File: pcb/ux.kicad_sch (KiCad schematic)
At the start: 41 parts, among them J5 Conn_01x40, J7 GameBoy_LinkPort, J8 Conn_01x02, SW12 A, SW13 B, SW14 START, SW15 SELECT, SW2 BOOT, SW3 RESET, SW4 UP, SW5 DOWN, SW6 LEFT, SW7 RIGHT, U5 APA2502, U7 ICM-42670-P, U8 TCA9535RTWR

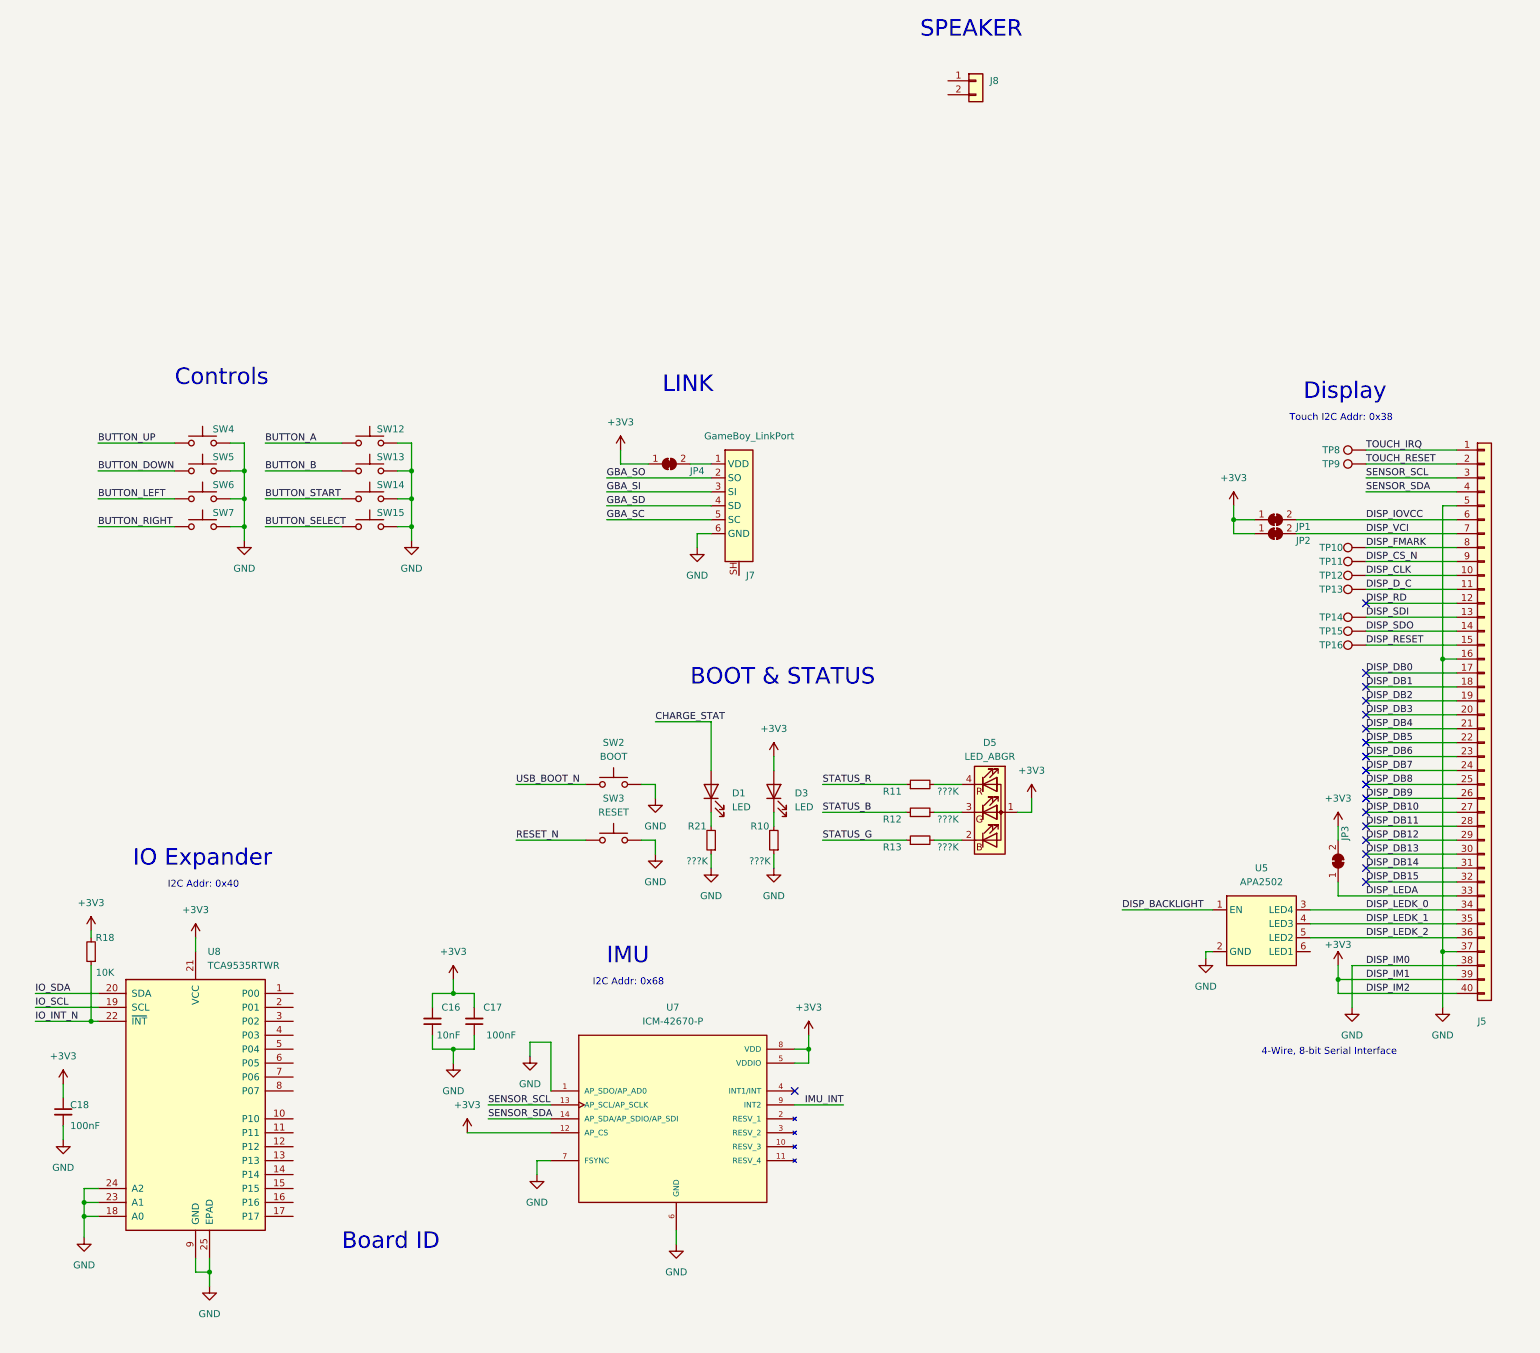
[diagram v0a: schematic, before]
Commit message: pcb: Update schematic to WIP6
Change-Id: I9e9f727ad2774ee986f2f97450dc509901129aec
Reviewed-on: https://pigweed-review.googlesource.com/c/pigweed/kudzu/+/169650
Reviewed-by: Anthony DiGirolamo <tonymd@google.com>
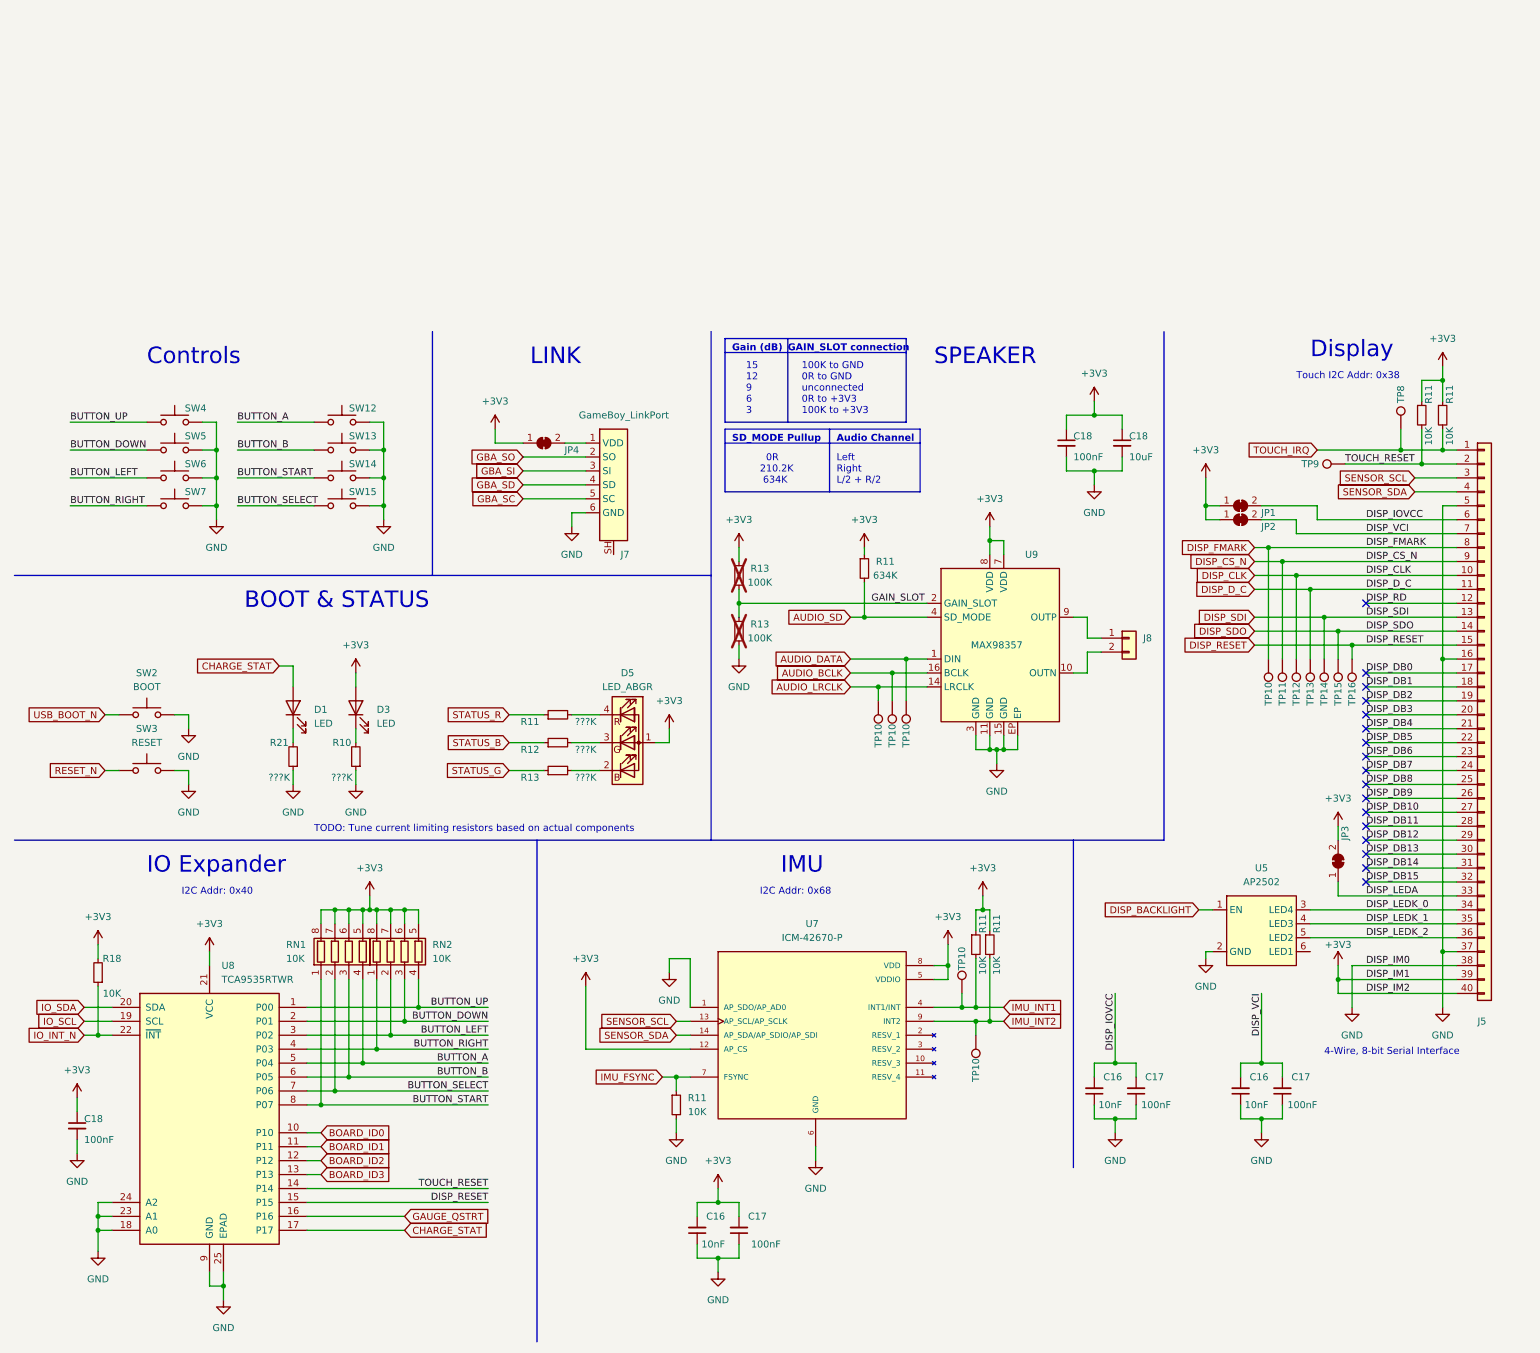
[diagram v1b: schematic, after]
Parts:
- added C16 (x2): 10nF, symbol Device:C_Small
- added C17 (x2), C18: 100nF, symbol Device:C_Small
- added C18: 10uF, symbol Device:C_Small
- added R11 (x5): 10K, symbol Device:R_Small
- added R11: 634K, symbol Device:R_Small
- added R13 (x2): 100K, symbol Device:R_Small
- added RN1, RN2: 10K, Resistor_THT:R_Array_SIP5, symbol Device:R_Pack04
- added TP10 (x5): RUN, symbol Connector:TestPoint
- added U9: MAX98357, symbol kudzu-parts:MAX98357
- D5: Price @ 10 (none) -> 0.07800; Price @ 25 (none) -> 0.07220
- J5: Price @ 10 (none) -> 0.17; Price @ 25 (none) -> 0.17
- J7: Price @ 10 (none) -> 2.09; Price @ 25 (none) -> 2.09
- U5: value APA2502 -> AP2502; DigiKey PN (none) -> AP2502KTR-G1DITR-ND; Price @ 10 (none) -> 0.34400; Price @ 25 (none) -> 0.32080
- U7: DigiKey PN (none) -> 1428-ICM-42670-PCT-ND; Price @ 10 (none) -> 3.66400; Price @ 25 (none) -> 3.25680
- U8: DigiKey PN (none) -> 296-25156-2-ND; Price @ 10 (none) -> 1.09300; Price @ 25 (none) -> 1.03800
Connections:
- net +3V3: now also C18.1, C18.1, R11.1, R11.1, R11.1, R11.1, R11.1, R13.2, RN1.5 (R4.2), RN1.6 (R3.2), RN1.7 (R2.2), RN1.8 (R1.2), RN2.5 (R4.2), RN2.6 (R3.2), RN2.7 (R2.2), RN2.8 (R1.2), U9.7 (VDD), U9.8 (VDD)
- net BUTTON_A: now also U8.5 (P04), RN1.4 (R4.1)
- net BUTTON_B: now also U8.6 (P05), RN1.3 (R3.1)
- net BUTTON_DOWN: now also U8.2 (P01), RN2.3 (R3.1)
- net BUTTON_LEFT: now also U8.3 (P02), RN2.2 (R2.1)
- net BUTTON_RIGHT: now also U8.4 (P03), RN2.1 (R1.1)
- net BUTTON_SELECT: now also U8.7 (P06), RN1.2 (R2.1)
- net BUTTON_START: now also U8.8 (P07), RN1.1 (R1.1)
- net BUTTON_UP: now also U8.1 (P00), RN2.4 (R4.1)
- net CHARGE_STAT: now also U8.17 (P17)
- net DISP_IOVCC: now also C16.2, C17.2
- net DISP_RESET: now also U8.15 (P15)
- net DISP_VCI: now also C16.2, C17.2
- net GND: now also C16.1, C16.1, C17.1, C17.1, C18.2, C18.2, R11.2, R13.1, U9.11 (GND), U9.15 (GND), U9.3 (GND), U9.EP; no longer U7.7 (FSYNC)
- net TOUCH_IRQ: now also R11.2
- net TOUCH_RESET: now also U8.14 (P14), R11.2
- net IMU_INT1: now reaches U7.4 (INT1/INT)
- net IMU_INT1: now also R11.2, TP10.1
- net BOARD_ID0: now reaches U8.10 (P10)
- net BOARD_ID1: now reaches U8.11 (P11)
- net BOARD_ID2: now reaches U8.12 (P12)
- net BOARD_ID3: now reaches U8.13 (P13)
- net GAUGE_QSTRT: now reaches U8.16 (P16)
- net at J8.1 (Pin_1): now also U9.9 (OUTP)
- net at J8.2 (Pin_2): now also U9.10 (OUTN)
- net IMU_INT renamed IMU_INT2
- net IMU_INT2: now also R11.2, TP10.1
- new net AUDIO_BCLK: TP10.1, U9.16 (BCLK)
- new net AUDIO_DATA: TP10.1, U9.1 (DIN)
- new net AUDIO_LRCLK: TP10.1, U9.14 (LRCLK)
- new net AUDIO_SD: R11.2, U9.4 (SD_MODE)
- new net GAIN_SLOT: R13.1, R13.2, U9.2 (GAIN_SLOT)
- new net IMU_FSYNC: R11.1, U7.7 (FSYNC)
- no-connect marks 18 -> 17
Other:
- note added: "0R 210.2K 634K"
- note added: "100K to GND 0R to GND unconnected 0R to +3V3 100K to +3V3"
- note added: "15 12 9 6 3"
- note added: "Audio Channel"
- note added: "GAIN_SLOT connection"
- note added: "Gain (dB)"
- note added: "Left Right L/2 + R/2"
- note added: "SD_MODE Pullup"
- note added: "TODO: Tune current limiting resistors based on actual components"
- note removed: "Board ID"
- moved on the sheet: C16, C17, C18, D1, D3, D5, J7, J8, JP1, JP2, JP4, R10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
